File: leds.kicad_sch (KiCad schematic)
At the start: 72 parts, among them Q1 BSS138, Q10 BSS138, Q11 BSS138, Q12 BSS138, Q13 BSS138, Q14 BSS138, Q15 BSS138, Q16 BSS138, Q17 BSS138, Q18 BSS138, Q19 BSS138, Q2 BSS138, Q20 BSS138, Q21 BSS138, Q22 BSS138, Q23 BSS138, Q24 BSS138, Q3 BSS138, Q4 BSS138, Q5 BSS138, Q6 BSS138, Q7 BSS138, Q8 BSS138, Q9 BSS138

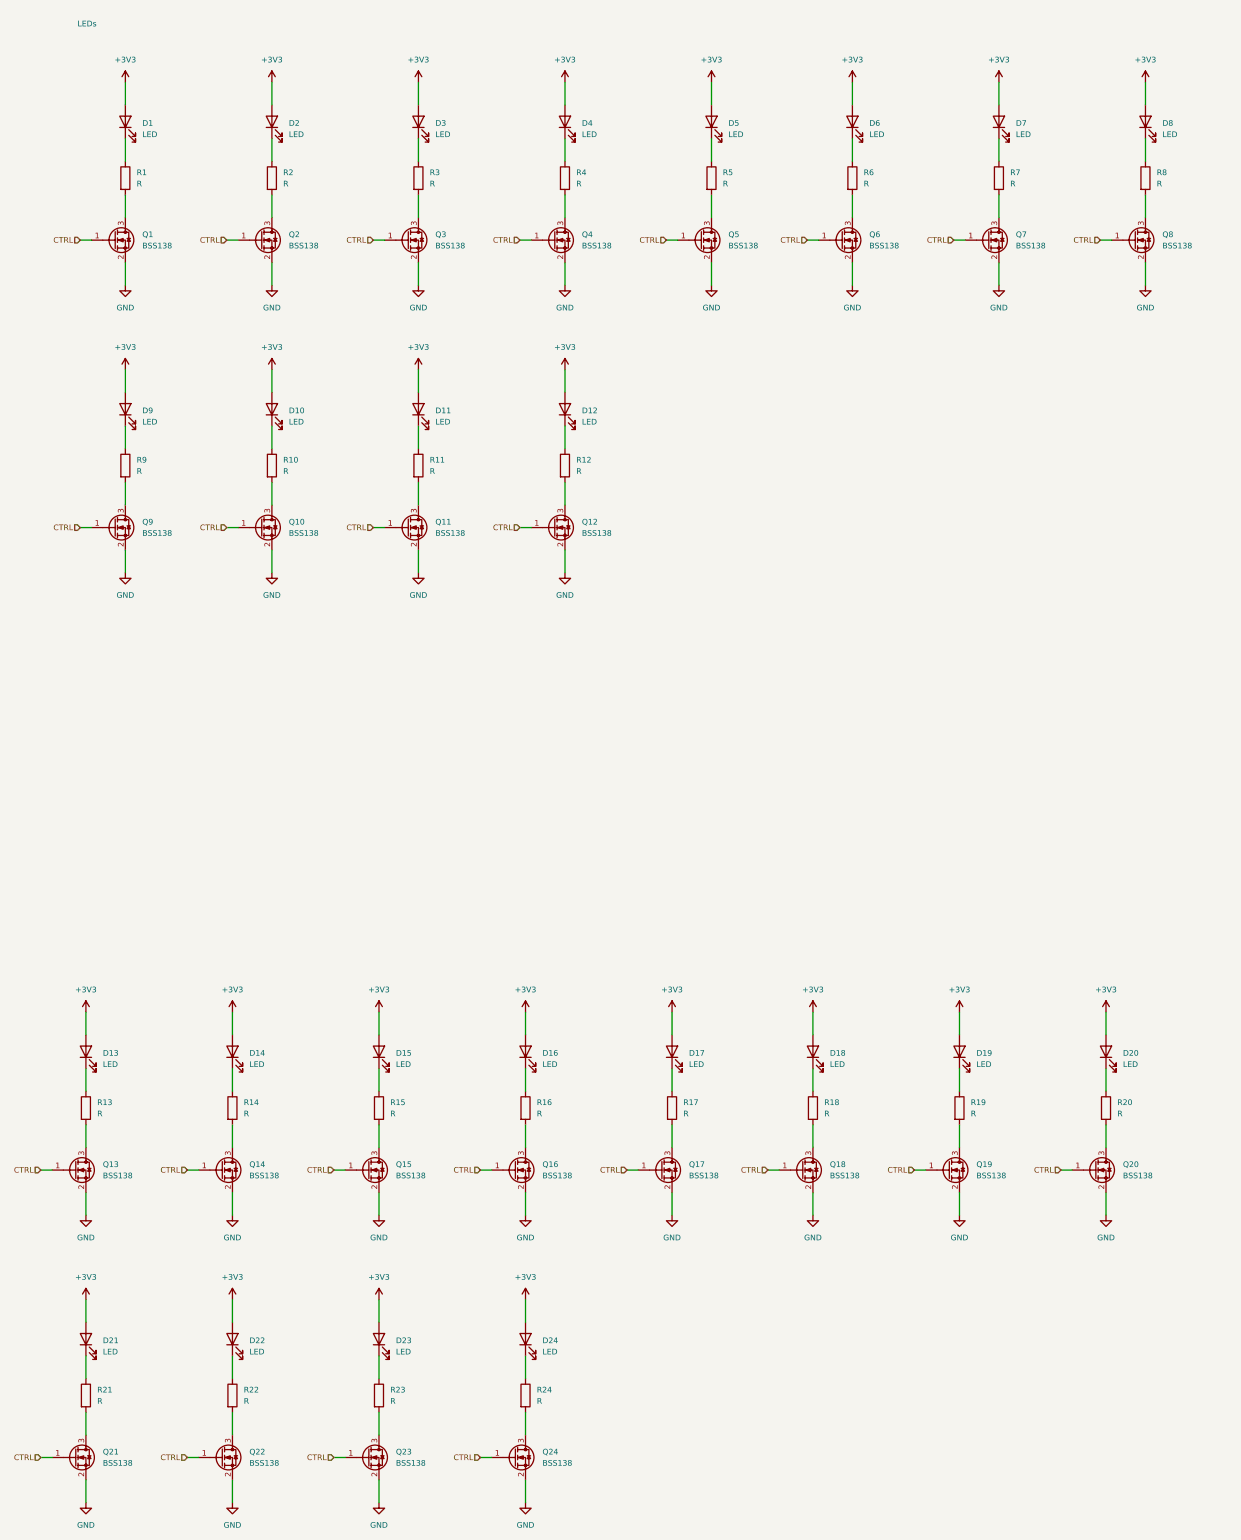
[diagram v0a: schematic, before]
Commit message: More routing
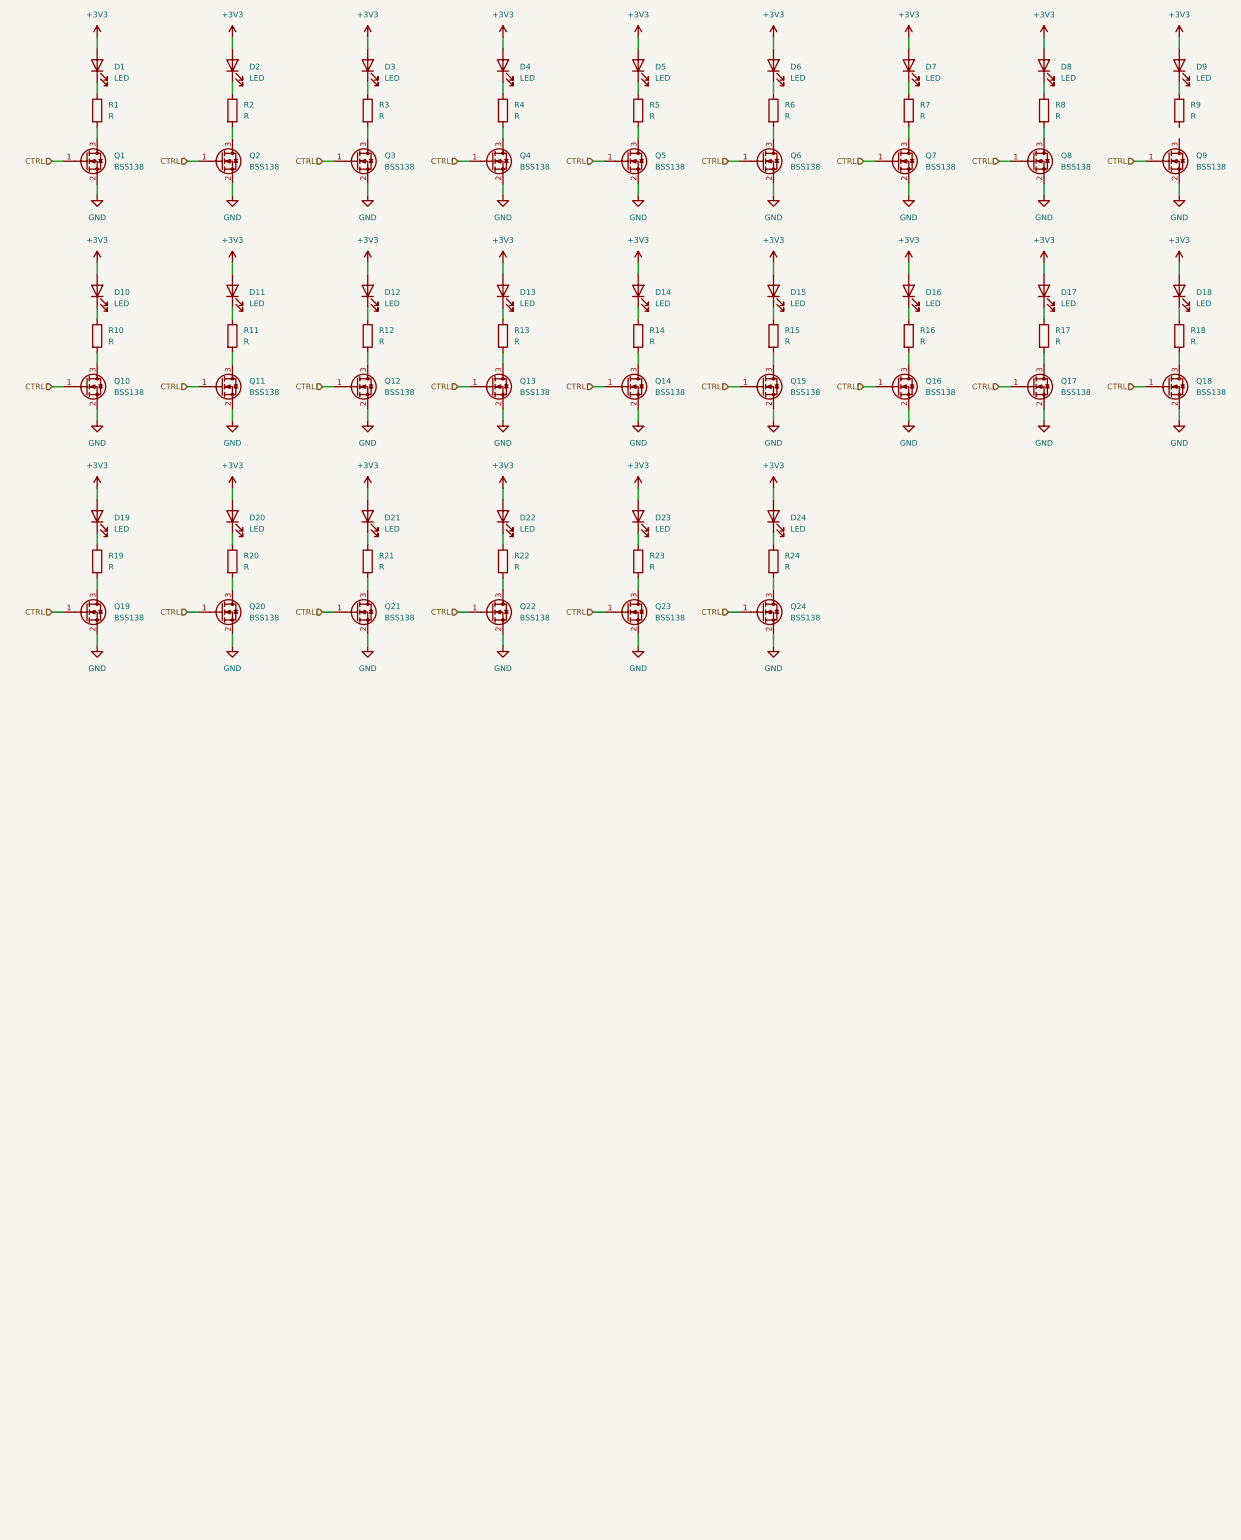
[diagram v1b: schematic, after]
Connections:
- net at R9.2: no longer Q9.3 (D)
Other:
- note removed: "LEDs"
- moved on the sheet: D1, D10, D11, D12, D13, D14, D15, D16, D17, D18, D19, D2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
